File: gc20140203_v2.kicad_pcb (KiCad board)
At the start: 6 copper layers, 173 parts, among them J1 JACK_2P, P1 USD, P10 CONN_1, P11 CONN_1, P2 Serial, P3 USB0, P4 USB1, P5 LCD_HEADER, P6 LAN_HEADER, P7 CONN_1, P8 CONN_1, P9 CONN_1, SW1 SW_PUSH, SW2 SW_PUSH, U1 TL5209D, U2 TPC65217C, U3 AM3359AZCZ100, U4 MT41K256M16HA-125:E, U5 SN74LVC2G241DCU, X1 24MHz, X2 CM200C

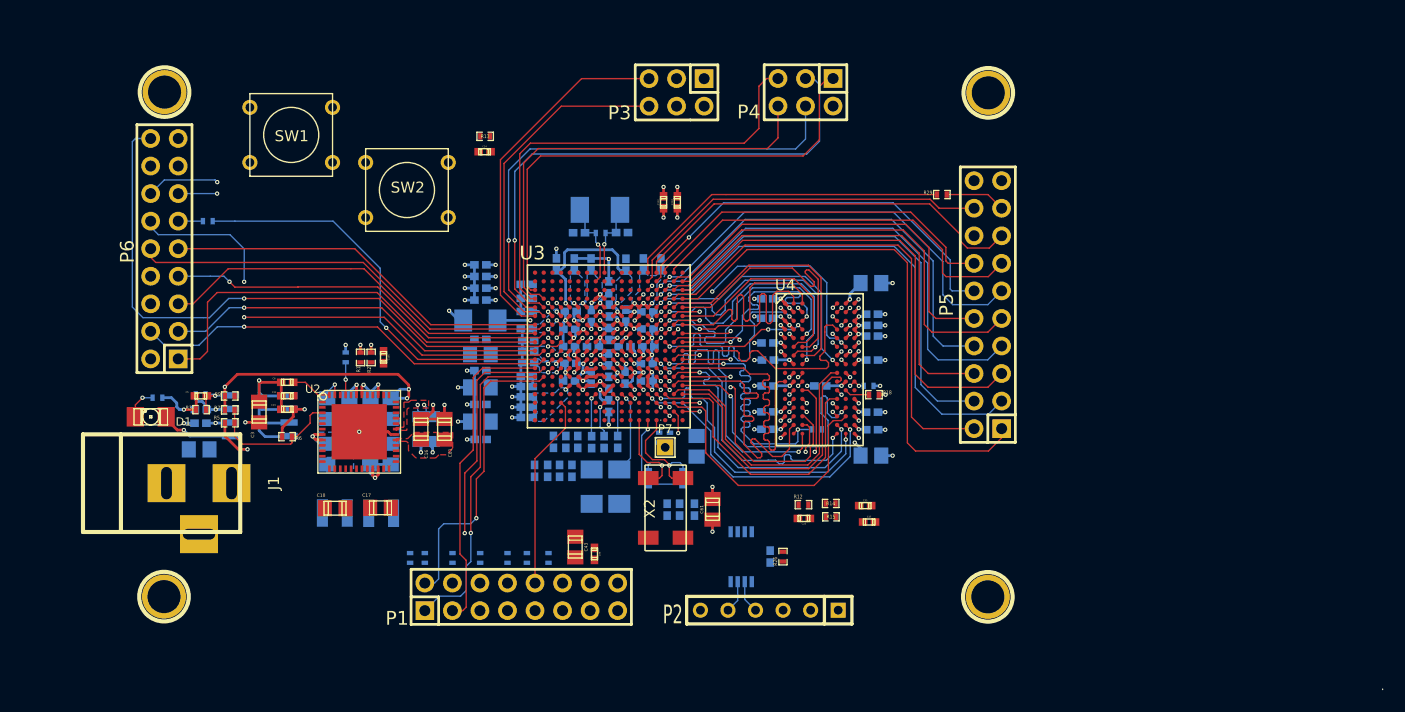
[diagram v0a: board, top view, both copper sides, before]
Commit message: Power supply
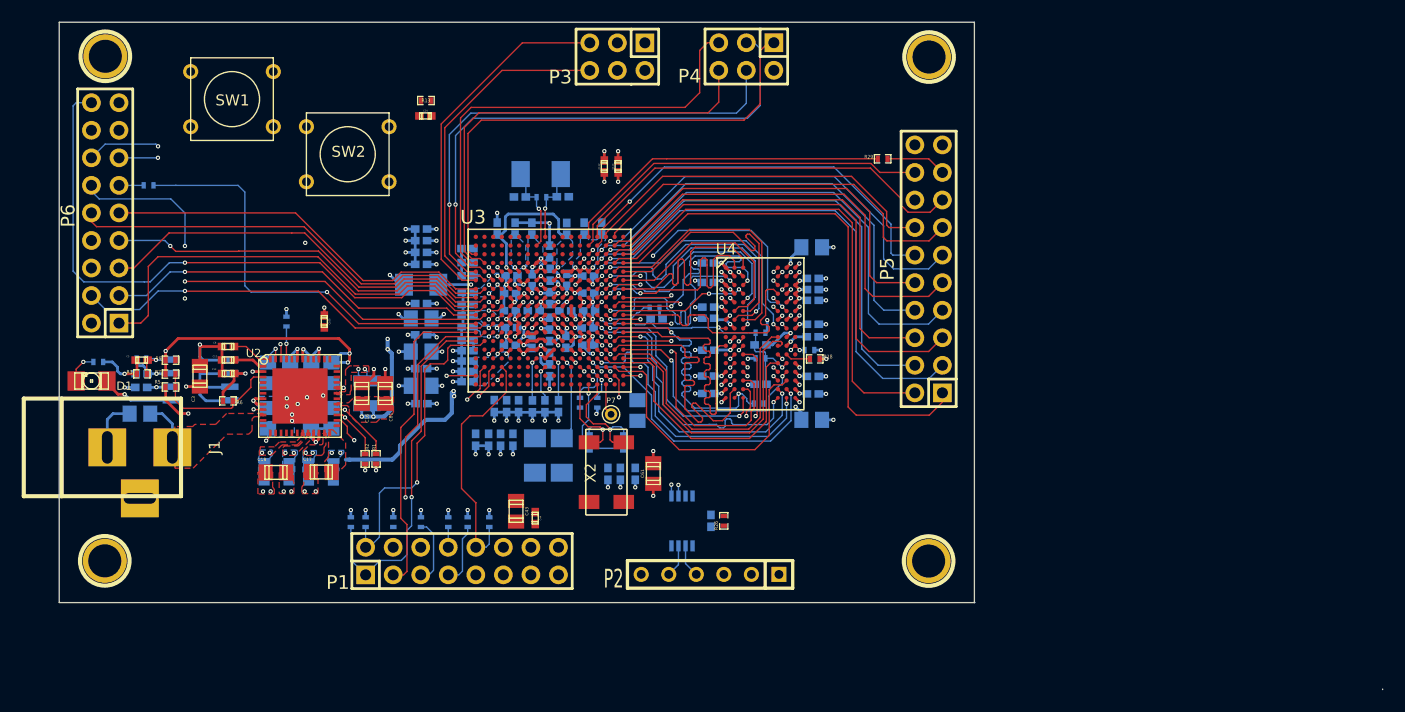
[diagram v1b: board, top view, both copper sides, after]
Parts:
- C23, C35, C37, R12, R14, R15: moved to B.Cu
- P7: footprint Connect:SIL-1 -> Connect:PINTST
- moved C23 22.9 mm to (158.7, 97.7)
- moved R12 22.7 mm to (158.5, 96.7)
- moved C35 17.7 mm to (168.2, 100.1), turned to 180 degrees
- moved R14 17.0 mm to (168.2, 99.0), turned to 180 degrees
- moved C37 16.2 mm to (168.2, 103.8)
- moved R15 16.0 mm to (168.2, 101.4), turned to 180 degrees
- moved R1 9.46 mm to (132.8, 110.6), turned to 90 degrees
- moved R2 9.38 mm to (131.8, 110.7), turned to 90 degrees
- moved R27 7.97 mm to (151.6, 105.5)
- moved R30 7.43 mm to (153.2, 105.5)
- moved L2 6.73 mm to (127.7, 111.8)
- moved C41 6.72 mm to (163.4, 97.7)
- moved L1 6.58 mm to (123.6, 111.8)
- moved C72 6.50 mm to (141.2, 96.4)
- moved C54 6.50 mm to (141.2, 98.5)
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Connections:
- C23 pad 1: Net-(C23-Pad1) -> +0.675V
- J1 pad 1: DGND -> +5V
- J1 pad 2: Net-(J1-Pad2) -> DGND
- J1 pad 3: +5V -> DGND
- U3 pad J4: Net-(C23-Pad1) -> +0.675V
- U3 pad P9: +1.8V -> (no net)
- X2 pad 1: Net-(C21-Pad2) -> Net-(C22-Pad2)
- X2 pad 4: Net-(C22-Pad2) -> Net-(C21-Pad2)
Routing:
- net /processor2/MII1_TXEN: track 7.39 -> 50.8 mm, vias 1 -> 2
- net /processor2/WAKEUP: track 0.00 -> 42.2 mm, vias 0 -> 2
- net /processor2/PMIC_POWER_EN: track 0.00 -> 39.5 mm, vias 0 -> 2
- net +5V: track 17.3 -> 52.0 mm, vias 6 -> 8
- net DGND: track 141.9 -> 176.2 mm, vias 85 -> 109
- net /processor1/LDO_PGOOD: track 0.00 -> 32.4 mm, vias 0 -> 2
- net /processor1/PMIC_PGOOD: track 0.00 -> 29.6 mm, vias 0 -> 2
- net Net-(U3-PadE15): track 0.00 -> 29.2 mm, vias 0 -> 2
- net Net-(U3-PadE16): track 0.00 -> 28.7 mm, vias 0 -> 2
- net /processor1/PMIC_INT: track 3.01 -> 29.1 mm, vias 1 -> 2
- net +0.675V: track 0.00 -> 25.0 mm, vias 0 -> 3
- net /processor2/I2C0_SCL: track 0.00 -> 23.5 mm, vias 0 -> 2
- net /processor2/I2C0_SDA: track 0.00 -> 21.6 mm, vias 0 -> 2
- net +1.1V: track 32.7 -> 49.2 mm, vias 19 -> 28
- net (no net): track 0.68 -> 15.7 mm, vias 1 -> 18
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- added copper zone on B.Cu, net +1.1V
- added copper zone on Inner2.Cu, net +1.1V
- added copper zone on B.Cu, net +1.35V
- added copper zone on F.Cu, net +1.35V
- added copper zone on Inner3.Cu, net +1.8V
- added copper zone on F.Cu, net +5V
- added copper zone on F.Cu, net DGND
- added copper zone on F.Cu, net Net-(L1-Pad1)
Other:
- board outline added: 122 x 61.5 mm

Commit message: PWR layer
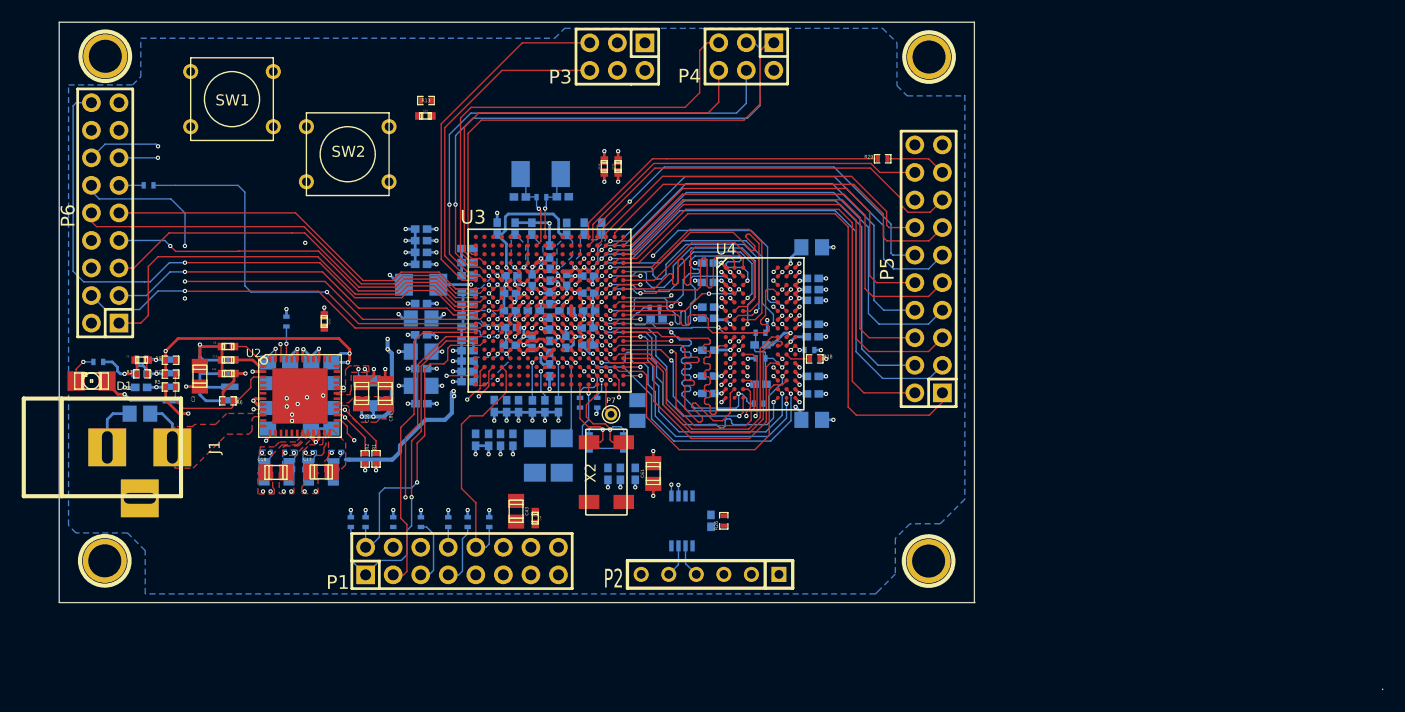
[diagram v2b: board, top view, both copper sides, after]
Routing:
- net Net-(C21-Pad2): track 11.2 -> 10.2 mm
- net Net-(C22-Pad2): track 9.46 -> 10.5 mm
- added copper zone on PWR.Cu, net +1.35V
- added copper zone on PWR.Cu, net +1.8V
- added copper zone on PWR.Cu, net 3V3
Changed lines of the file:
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@@
   (general
     (links 636)
-    (no_connects 304)
-    (area 105.451879 72.5528 225.650001 131.960001)
+    (no_connects 307)
+    (area 99.991879 69.2528 225.650001 131.960001)
     (thickness 1.6)
     (drawings 7)
@@
   (page A4)
   (layers
-    (15 F.Cu signal)
-    (4 GND.Cu power)
-    (3 Inner3.Cu signal)
-    (2 Inner2.Cu signal)
+    (15 F.Cu signal hide)
+    (4 GND.Cu power hide)
+    (3 Inner3.Cu signal hide)
+    (2 Inner2.Cu signal hide)
     (1 PWR.Cu power)
-    (0 B.Cu signal)
+    (0 B.Cu signal hide)
     (16 B.Adhes user)
     (17 F.Adhes user)
@@
   (segment (start 126.03146 101.44148) (end 126.03146 100.58854) (width 0.254) (layer F.Cu) (net 1))
   (via (at 115.28 103.97) (size 0.4) (layers F.Cu B.Cu) (net 1))
-  (segment (start 173.60864 103.03) (end 174.28 103.03) (width 0.381) (layer B.Cu) (net 2) (status 400000))
+  (segment (start 173.60864 103.03) (end 174.28 103.03) (width 0.381) (layer B.Cu) (net 2))
   (via (at 174.28 103.03) (size 0.4) (layers F.Cu B.Cu) (net 2))
   (segment (start 124.87 104.84) (end 125.78 104.84) (width 0.127) (layer F.Cu) (net 2))
@@
   (segment (start 152.65 107.67) (end 152.43 107.89) (width 0.127) (layer B.Cu) (net 13))
   (segment (start 152.35 107.68) (end 151.59 106.92) (width 0.127) (layer F.Cu) (net 13))
-  (via (at 154.37 107.94) (size 0.4) (layers F.Cu B.Cu) (net 13))
   (segment (start 153.43 107.67) (end 152.65 107.67) (width 0.127) (layer B.Cu) (net 13))
   (segment (start 153.44 107.68) (end 152.35 107.68) (width 0.127) (layer F.Cu) (net 13))
+  (via (at 154.37 107.94) (size 0.4) (layers F.Cu B.Cu) (net 13))
   (segment (start 154.37 107.94) (end 154.37 107.86) (width 0.127) (layer F.Cu) (net 13))
-  (segment (start 154.37 107.94) (end 154.63 107.68) (width 0.127) (layer B.Cu) (net 13))
-  (segment (start 154.37 107.86) (end 153.92 107.41) (width 0.127) (layer F.Cu) (net 13))
   (segment (start 153.7 107.94) (end 153.43 107.67) (width 0.127) (layer B.Cu) (net 13))
   (segment (start 153.7 107.94) (end 153.44 107.68) (width 0.127) (layer F.Cu) (net 13))
@@
   (segment (start 153.19 104.64) (end 153.19 103.77) (width 0.127) (layer F.Cu) (net 14))
   (segment (start 152.43 109.11) (end 153.47 109.11) (width 0.127) (layer F.Cu) (net 14))
+  (segment (start 154.37 107.94) (end 154.63 107.68) (width 0.127) (layer B.Cu) (net 14))
+  (segment (start 154.37 107.86) (end 153.92 107.41) (width 0.127) (layer F.Cu) (net 14))
   (segment (start 170.24 102.21) (end 169.4 101.37) (width 0.127) (layer B.Cu) (net 16))
   (via (at 170.24 102.21) (size 0.4) (layers F.Cu B.Cu) (net 16))
@@
     (polygon
       (pts
-        (xy 122.82 107.2) (xy 123.64 107.2) (xy 124.34 107.2) (xy 124.34 104.88) (xy 121.97 104.88)
-        (xy 121.97 103.59) (xy 129.5 103.59) (xy 129.5 105.96) (xy 125.26 105.96) (xy 125.26 108.64)
-        (xy 122.81 108.64) (xy 122.81 107.2) (xy 122.82 107.2)
+        (xy 187.08 114.35) (xy 184.81 116.62) (xy 182.02 116.62) (xy 180.67 117.97) (xy 180.67 121.26)
+        (xy 179.2 122.73) (xy 178.84 123.09) (xy 111.51 123.09) (xy 111.51 119.1) (xy 109.88 117.47)
+        (xy 105.13 117.47) (xy 104.44 116.78) (xy 104.44 76.16) (xy 110.34 76.16) (xy 111.1 75.4)
+        (xy 111.1 71.86) (xy 149.26 71.86) (xy 150.18 70.94) (xy 179.49 70.94) (xy 180.82 72.27)
+        (xy 180.82 76.23) (xy 181.76 77.17) (xy 187.07 77.17) (xy 187.08 77.11) (xy 187.08 114.35)
       )
     )
@@
       )
     )
+  )
+  (zone (net 9) (net_name +1.35V) (layer PWR.Cu) (hatch edge 0.508)
+    (connect_pads yes (clearance 0.1))
+    (min_thickness 0.127)
+    (fill (arc_segments 16) (thermal_gap 0.1) (thermal_bridge_width 0.254))
+    (polygon
+      (pts
+        (xy 175.87 108.13) (xy 174.96 109.04) (xy 164.4 109.04) (xy 162.67 110.77) (xy 157.63 110.77)
+        (xy 157.63 107.16) (xy 156.08 105.61) (xy 156.08 104.2) (xy 152.4 100.52) (xy 152.4 95.32)
+        (xy 152.39 95.32) (xy 152.77 94.94) (xy 153.35 94.94) (xy 153.6 94.69) (xy 153.6 92.91)
+        (xy 155.09 91.42) (xy 162.42 91.42) (xy 164.46 89.38) (xy 175.11 89.38) (xy 175.87 90.14)
+      )
+    )
+  )
+  (zone (net 7) (net_name +1.8V) (layer PWR.Cu) (hatch edge 0.508)
+    (connect_pads yes (clearance 0.1))
+    (min_thickness 0.127)
+    (fill (arc_segments 16) (thermal_gap 0.1) (thermal_bridge_width 0.254))
+    (polygon
+      (pts
+        (xy 129.86 102.09) (xy 130.71 102.09) (xy 132.55 100.25) (xy 132.55 96.33) (xy 134.69 94.19)
+        (xy 134.69 92.81) (xy 132.37 92.81) (xy 130.12 95.06) (xy 130.12 99.36) (xy 129.75 99.73)
+        (xy 129.75 102.09) (xy 129.86 102.09)
+      )
+    )
+  )
+  (zone (net 7) (net_name +1.8V) (layer PWR.Cu) (hatch edge 0.508)
+    (connect_pads yes (clearance 0.1))
+    (min_thickness 0.127)
+    (fill (arc_segments 16) (thermal_gap 0.1) (thermal_bridge_width 0.254))
+    (polygon
+      (pts
+        (xy 150.9 101.22) (xy 151.36 101.22) (xy 151.58 101) (xy 151.58 100.69) (xy 151.69 100.58)
+        (xy 152.23 100.58) (xy 152.23 96.98) (xy 144.4 96.98) (xy 144.17 97.21) (xy 143.62 97.76)
+        (xy 143.62 98.74) (xy 143.76 98.88) (xy 149.51 98.88) (xy 149.76 99.13) (xy 150.33 99.13)
+        (xy 150.33 100.44) (xy 150.33 100.77) (xy 150.78 101.22) (xy 150.9 101.22)
+      )
+    )
+  )
+  (zone (net 7) (net_name +1.8V) (layer PWR.Cu) (hatch edge 0.508)
+    (connect_pads yes (clearance 0.1))
+    (min_thickness 0.127)
+    (fill (arc_segments 16) (thermal_gap 0.1) (thermal_bridge_width 0.254))
+    (polygon
+      (pts
+        (xy 150.23 100.58) (xy 145.21 100.58) (xy 145.21 101.27) (xy 144.39 101.27) (xy 144.39 99.01)
+        (xy 149.4 99.01) (xy 149.71 99.32) (xy 150.23 99.32)
+      )
+    )
+  )
+  (zone (net 7) (net_name +1.8V) (layer PWR.Cu) (hatch edge 0.508)
+    (connect_pads yes (clearance 0.1))
+    (min_thickness 0.127)
+    (fill (arc_segments 16) (thermal_gap 0.1) (thermal_bridge_width 0.254))
+    (polygon
+      (pts
+        (xy 147.6 100.7) (xy 149.38 100.7) (xy 149.99 101.31) (xy 149.99 110.57) (xy 147.68 110.57)
+        (xy 147.68 100.71) (xy 147.69 100.71)
+      )
+    )
+  )
+  (zone (net 6) (net_name 3V3) (layer PWR.Cu) (hatch edge 0.508)
+    (connect_pads yes (clearance 0.1))
+    (min_thickness 0.127)
+    (fill (arc_segments 16) (thermal_gap 0.1) (thermal_bridge_width 0.254))
+    (polygon
+      (pts
+        (xy 123.75 96.4) (xy 129.62 96.4) (xy 129.93 96.71) (xy 129.93 99.2) (xy 129.56 99.57)
+        (xy 129.56 102.27) (xy 130.86 102.27) (xy 132.64 100.49) (xy 132.84 100.29) (xy 132.84 96.42)
+        (xy 134.79 94.47) (xy 134.79 87.63) (xy 141.08 81.34) (xy 161.57 81.34) (xy 163.34 83.11)
+        (xy 163.34 89.63) (xy 162.09 90.88) (xy 155.09 90.88) (xy 153.26 92.71) (xy 153.26 94.69)
+        (xy 153.22 94.73) (xy 152.43 94.73) (xy 152.19 94.97) (xy 152.19 96.55) (xy 152.01 96.73)
+        (xy 144.34 96.73) (xy 143.48 97.59) (xy 143.48 98.7) (xy 143.48 98.72) (xy 143.48 99)
+        (xy 143.65 99.17) (xy 144.2 99.17) (xy 144.2 101.36) (xy 144.28 101.44) (xy 145.28 101.44)
+        (xy 145.4 101.32) (xy 145.4 100.82) (xy 145.5 100.72) (xy 147.33 100.72) (xy 147.53 100.92)
+        (xy 147.53 113.28) (xy 151.31 117.06) (xy 151.13 117.24) (xy 129.81 117.24) (xy 129.81 109.31)
+        (xy 123.75 109.31) (xy 123.75 96.41) (xy 123.76 96.41)
+      )
+    )

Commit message: GND layer
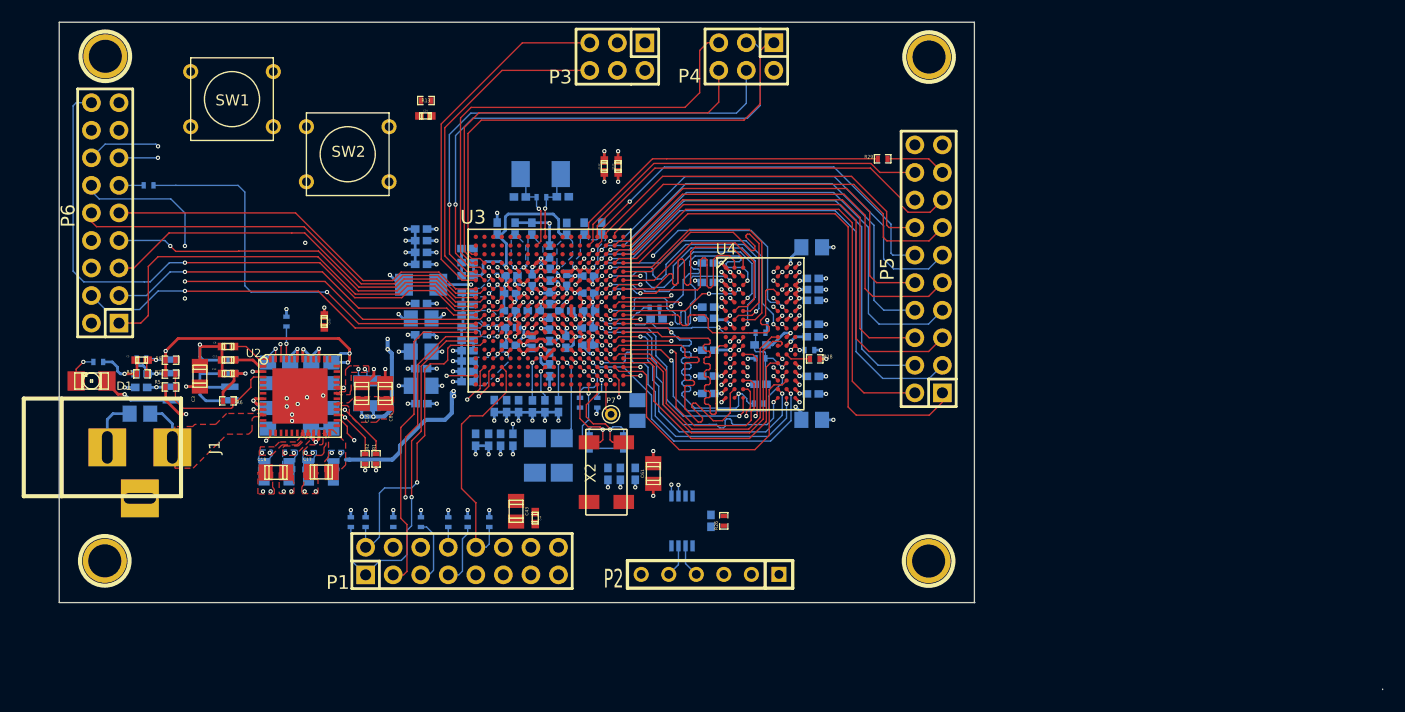
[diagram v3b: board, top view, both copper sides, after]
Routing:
- net Net-(C92-Pad1): track 0.00 -> 12.6 mm, vias 0 -> 2
- net +1.8V: track 61.1 -> 66.7 mm, vias 19 -> 20
- net Net-(C22-Pad2): track 10.5 -> 7.46 mm, vias 1 -> 0
- net Net-(C21-Pad2): track 10.2 -> 13.2 mm, vias 1 -> 2
- net (no net): track 15.7 -> 15.0 mm, vias 18 -> 17
- added copper zone on PWR.Cu, net DGND
- removed copper zone on B.Cu, net DGND
